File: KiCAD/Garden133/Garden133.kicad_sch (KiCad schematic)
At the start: 24 parts, among them U1 SHTC3, U2 RFM95W-915S2, U3 NCP114ASN330T1G

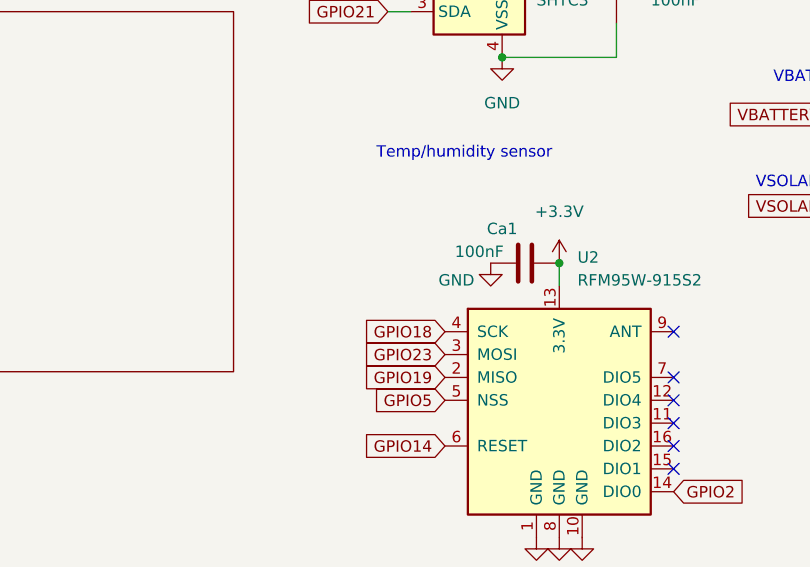
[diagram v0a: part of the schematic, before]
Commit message: Garden133 Board v6.2 (ordered from PCBWay)
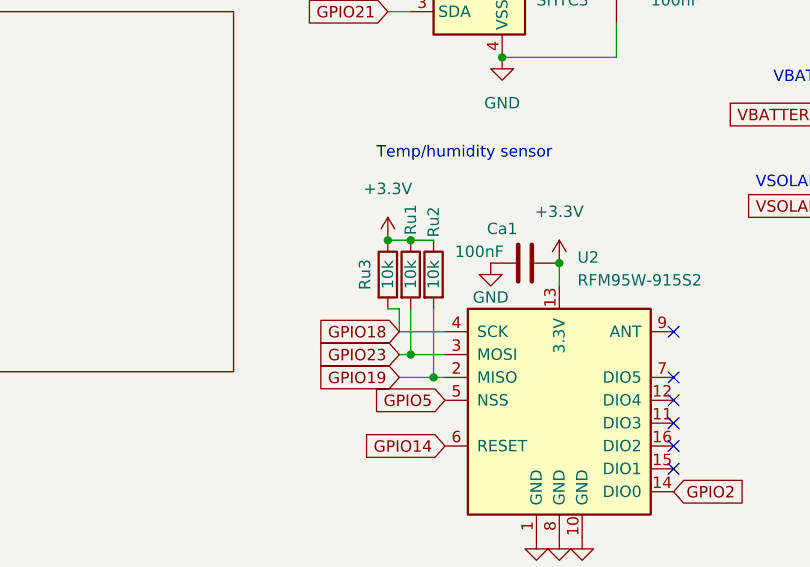
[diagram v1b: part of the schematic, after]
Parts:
- added Ru1, Ru2, Ru3: 10k, Resistor_SMD:R_0603_1608Metric, symbol Device:R
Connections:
- net +3.3V: now also Ru1.1, Ru2.1, Ru3.1
- net GPIO18: now also Ru3.2
- net GPIO19: now also Ru2.2
- net GPIO23: now also Ru1.2
